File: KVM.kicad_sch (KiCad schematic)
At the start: 3 parts, among them SW1 SW_SPDT

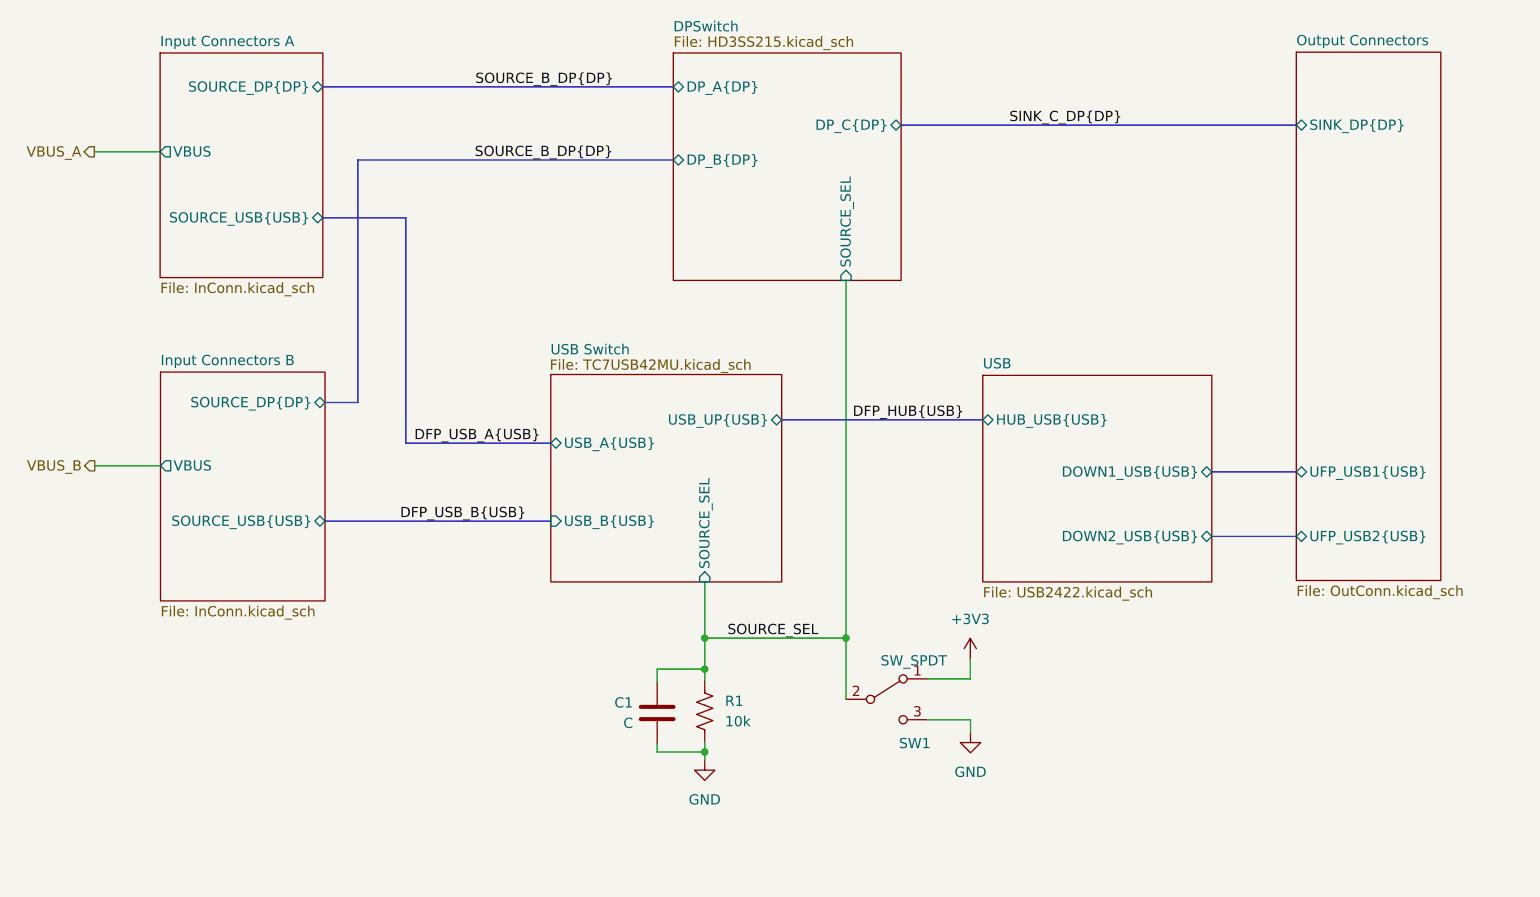
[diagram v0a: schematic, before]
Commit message: Pushing what i have now
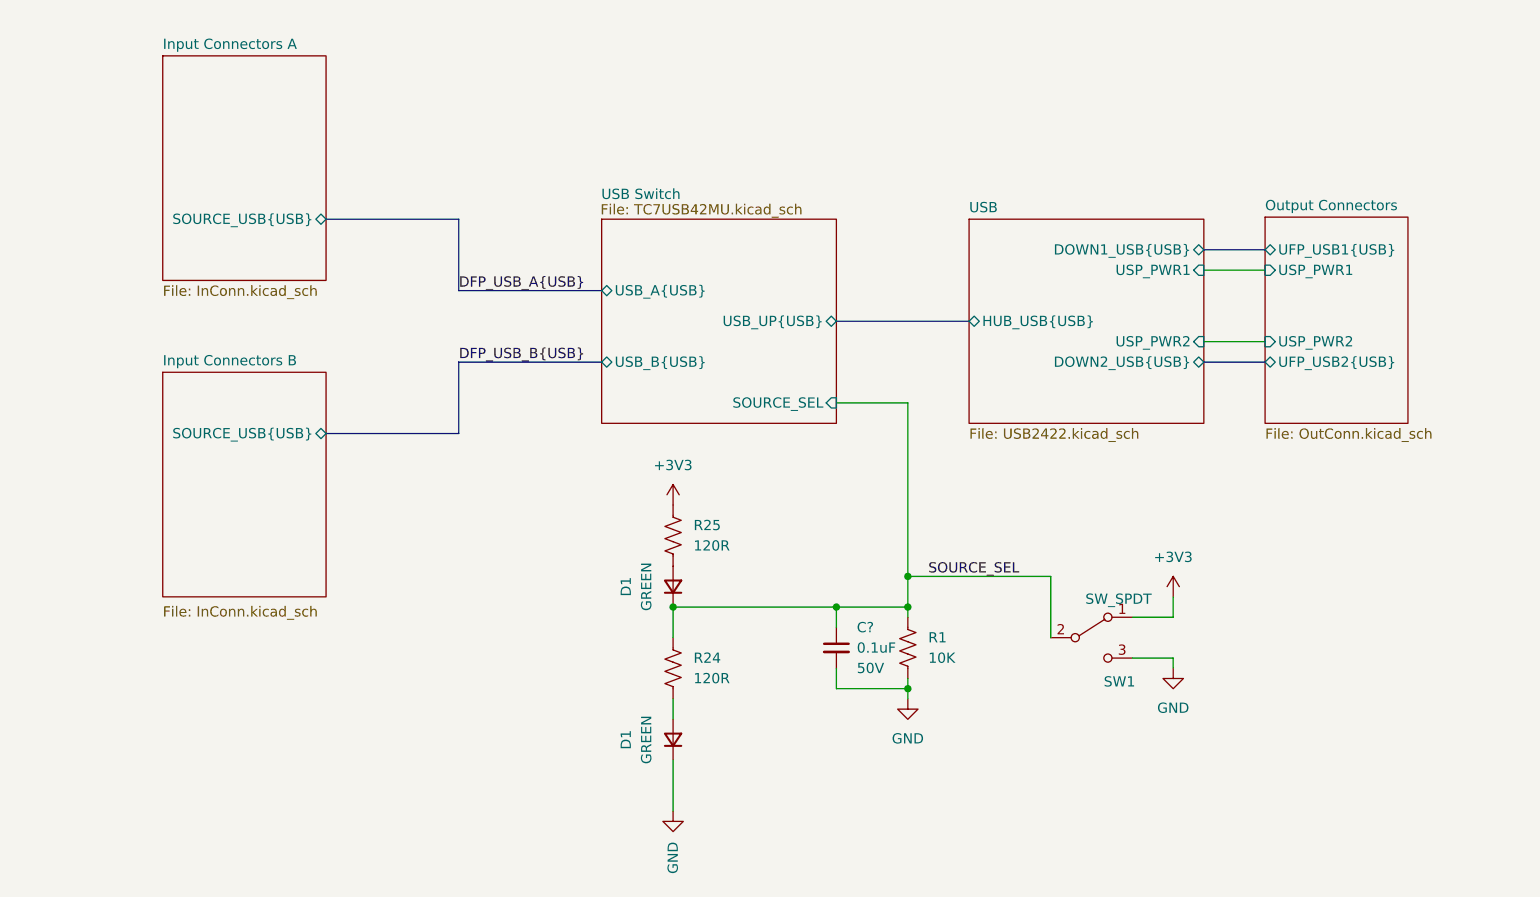
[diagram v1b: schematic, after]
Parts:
- removed C1: C, symbol Device:C
- removed R1: 10k, symbol Device:R_US
- added C?: ${Capacitance}, Capacitor_SMD:C_0603_1608Metric_Pad1.08x0.95mm_HandSolder, symbol Rockerrobotics:Capacitors/1276-1935-1-ND
- added D1 (x2): ${Color}, Diode_SMD:D_0805_2012Metric_Pad1.15x1.40mm_HandSolder, symbol Rockerrobotics:Diodes/754-2043-1-ND
- added R1: ${Resistance}, Resistor_SMD:R_0805_2012Metric_Pad1.20x1.40mm_HandSolder, symbol Rockerrobotics:Resistors/RNCP0805FTD10K0CT-ND
- added R24, R25: ${Resistance}, Resistor_SMD:R_0805_2012Metric_Pad1.20x1.40mm_HandSolder, symbol Rockerrobotics:Resistors/311-120ARCT-ND
- SW1: footprint (none) -> Connector_PinHeader_2.54mm:PinHeader_1x03_P2.54mm_Vertical
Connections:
- net +3V3: now also R25.1
- net GND: now also C?.2, D1.1 (K), R1.2
- net SOURCE_SEL: now also C?.1, D1.1 (K), R1.1, R24.1
- new net: D1.2 (A), R24.2
- new net: D1.2 (A), R25.2
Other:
- removed sheet DPSwitch
- sheet Input Connectors A ports: added none; removed SOURCE_DP{DP}, VBUS
- sheet Input Connectors B ports: added none; removed SOURCE_DP{DP}, VBUS
- sheet Output Connectors ports: added USP_PWR1, USP_PWR2; removed SINK_DP{DP}
- sheet USB ports: added USP_PWR1, USP_PWR2; removed none
- moved on the sheet: SW1
